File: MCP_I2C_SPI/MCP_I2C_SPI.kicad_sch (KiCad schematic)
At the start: 46 parts, among them J10 VCC, J11 GND, J21 V0, J22 Ext, J26 I2C, J3 Data, J30 Interrupt0, J34 A2, J35 SDA, J36 GPB, J37 GPA, J38 A1, J39 SCK, J4 Control, J40 A0, J41 INTA, J42 INTB, J43 SPI, J44 InterruptS, J45 A2, J46 GPB, J47 GPA, J48 A1, J49 A0, J5 Zlacze_LCD, J50 INTA, J51 INTB, J6 VSS, J7 K, J8 VDD, J9 A, U3 MCP23017_SP, U4 MCP23017_SP

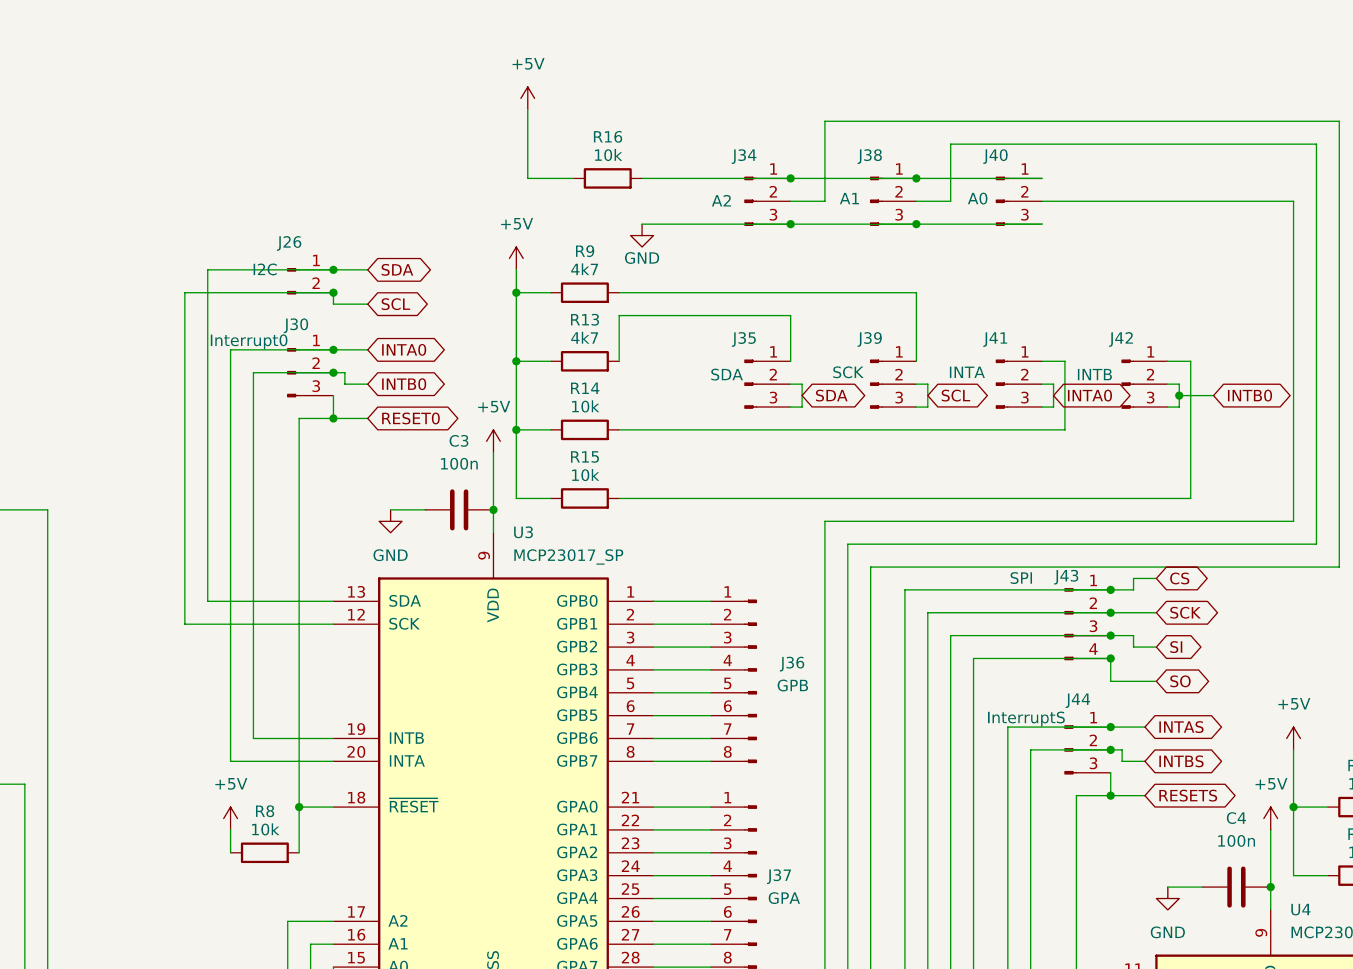
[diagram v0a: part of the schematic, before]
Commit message: MCP_I2C_SPI_PCB_V6
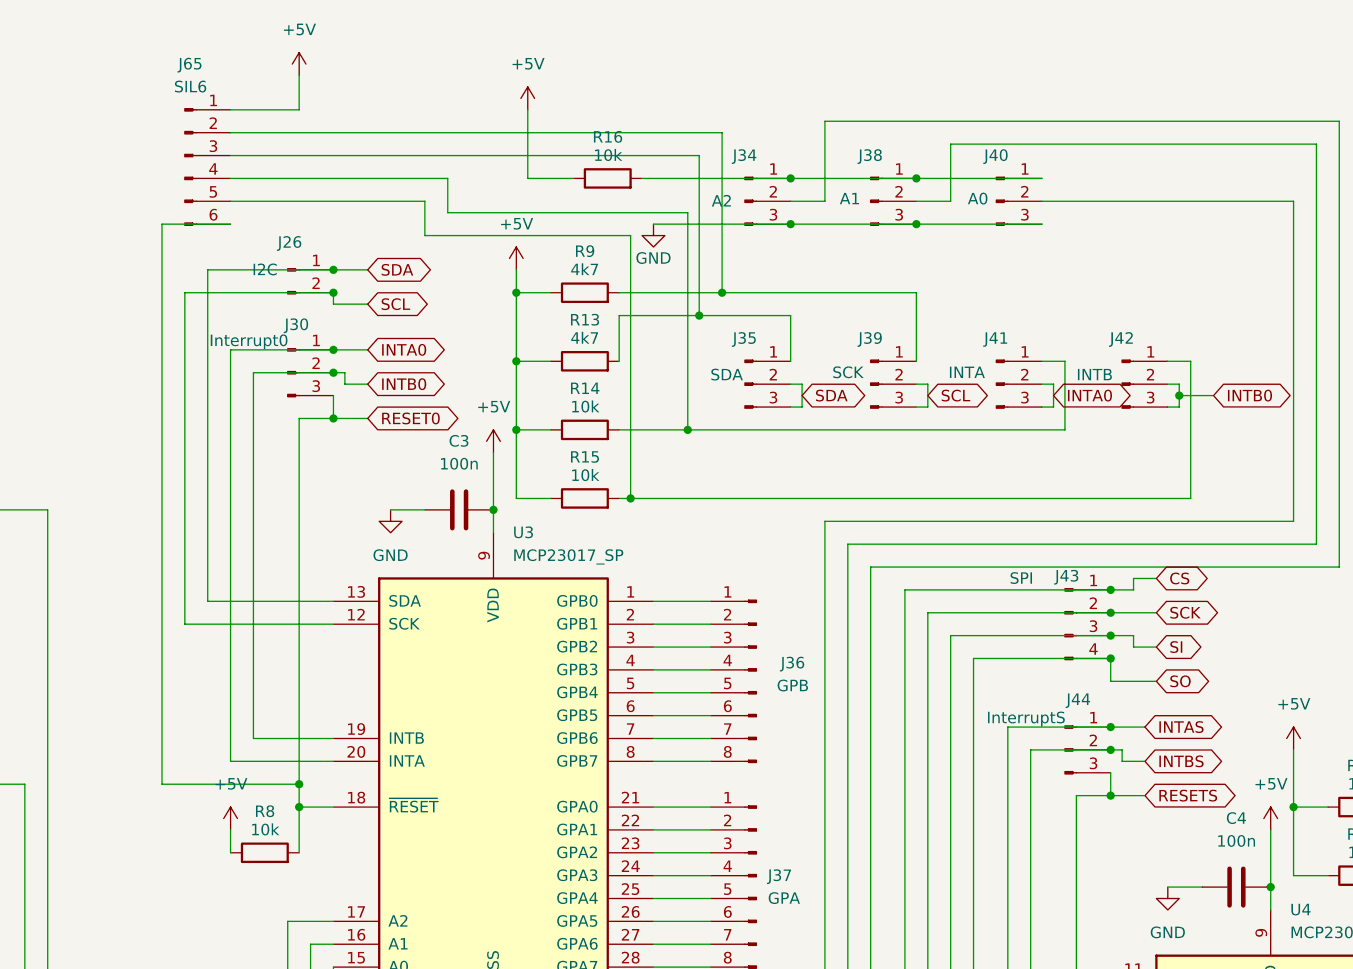
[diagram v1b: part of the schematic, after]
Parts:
- added J65: SIL6, Connector_PinSocket_2.54mm:PinSocket_1x06_P2.54mm_Vertical, symbol Connector:Conn_01x06_Pin
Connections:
- net +5V: now also J65.1 (Pin_1)
- net RESET0: now also J65.6 (Pin_6)
- net at J42.1 (Pin_1), R15.2: now also J65.5 (Pin_5)
- net at J41.1 (Pin_1), R14.2: now also J65.4 (Pin_4)
- net at J35.1 (Pin_1), R13.2: now also J65.3 (Pin_3)
- net at J39.1 (Pin_1), R9.2: now also J65.2 (Pin_2)
